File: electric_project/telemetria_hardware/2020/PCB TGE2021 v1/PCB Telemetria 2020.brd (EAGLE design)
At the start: 160 x 100 mm, 22 parts, among them IC1 INA240A1DR, IC2 MCP3221A6T-E_OTVAO, IC3 AZ1117IH-3.3TRG1, IC4 ACS758LCB-050B-PFF-T

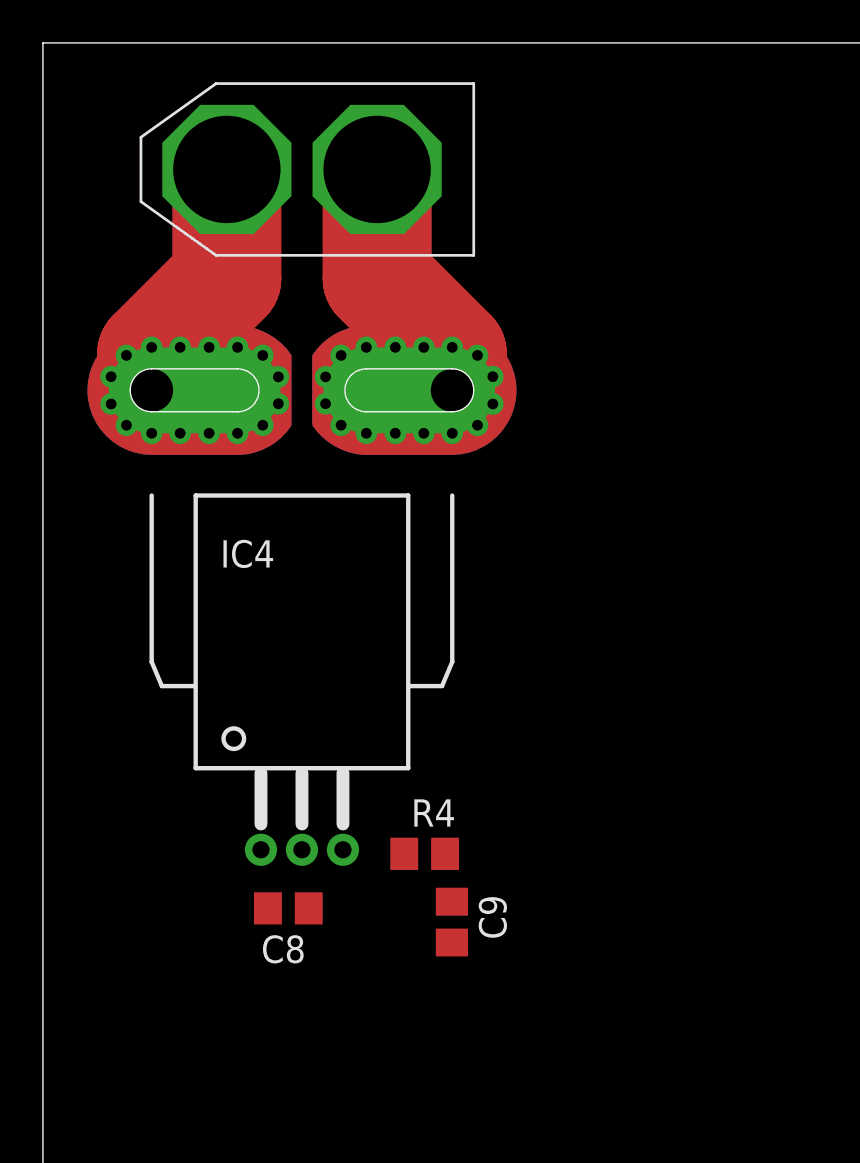
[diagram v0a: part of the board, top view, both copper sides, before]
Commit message: XT60 changes
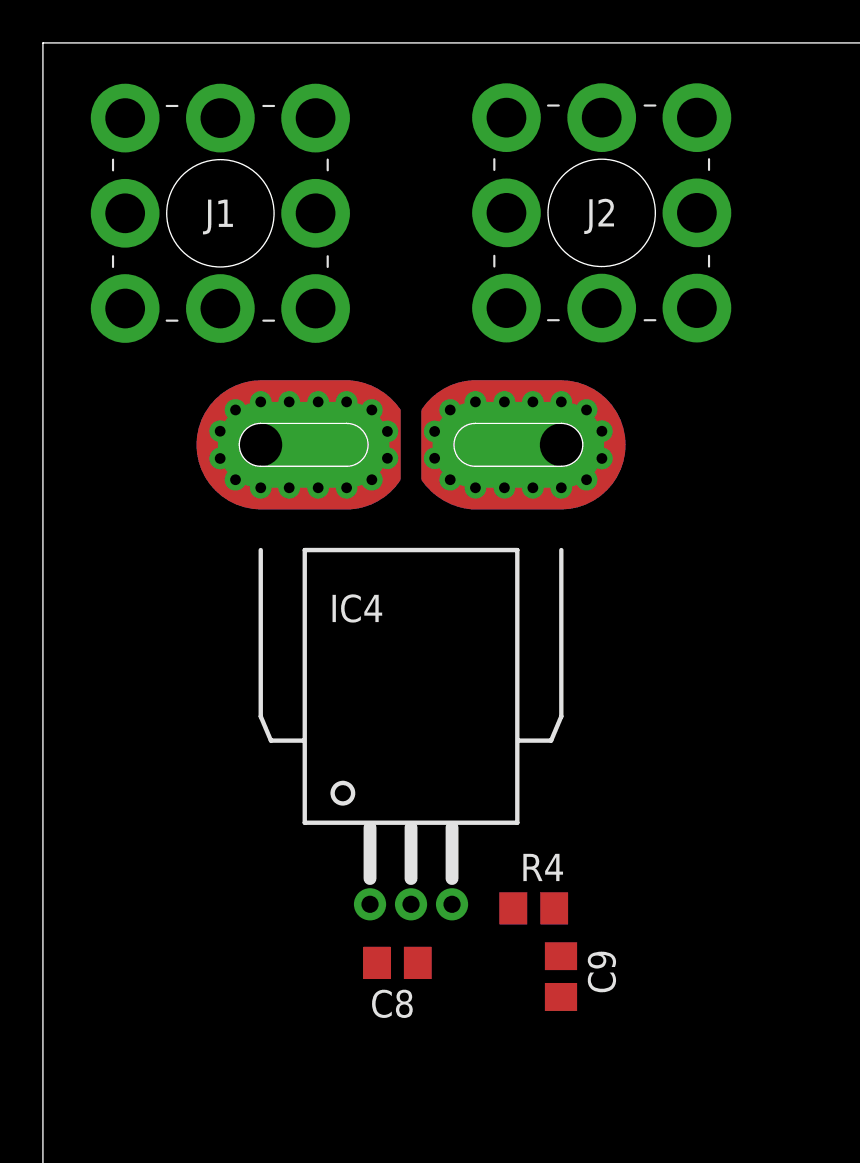
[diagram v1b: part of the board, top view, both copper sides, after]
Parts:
- removed U$3: XT60, XT60:XT60
- added J1, J2: 74655095R, SamacSys_Parts:74655095R
- moved C8 5.68 mm to (16.5, 57.1)
- moved C9 5.68 mm to (24.1, 56.5)
- moved R4 5.68 mm to (22.9, 59.7)
- moved IC4 5.68 mm to (17.1, 81.3)
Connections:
- net CMPPT_M: now also J1.1, J1.2, J1.3, J1.4, J1.5, J1.6, J1.7, J1.8; no longer U$3.-
- net CMPPT_P: now also J2.1, J2.2, J2.3, J2.4, J2.5, J2.6, J2.7, J2.8; no longer U$3.+
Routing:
- net CMPPT_M: track 11.7 -> 0.00 mm
- net CMPPT_P: track 11.7 -> 0.00 mm

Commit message: Adding XT60 documents
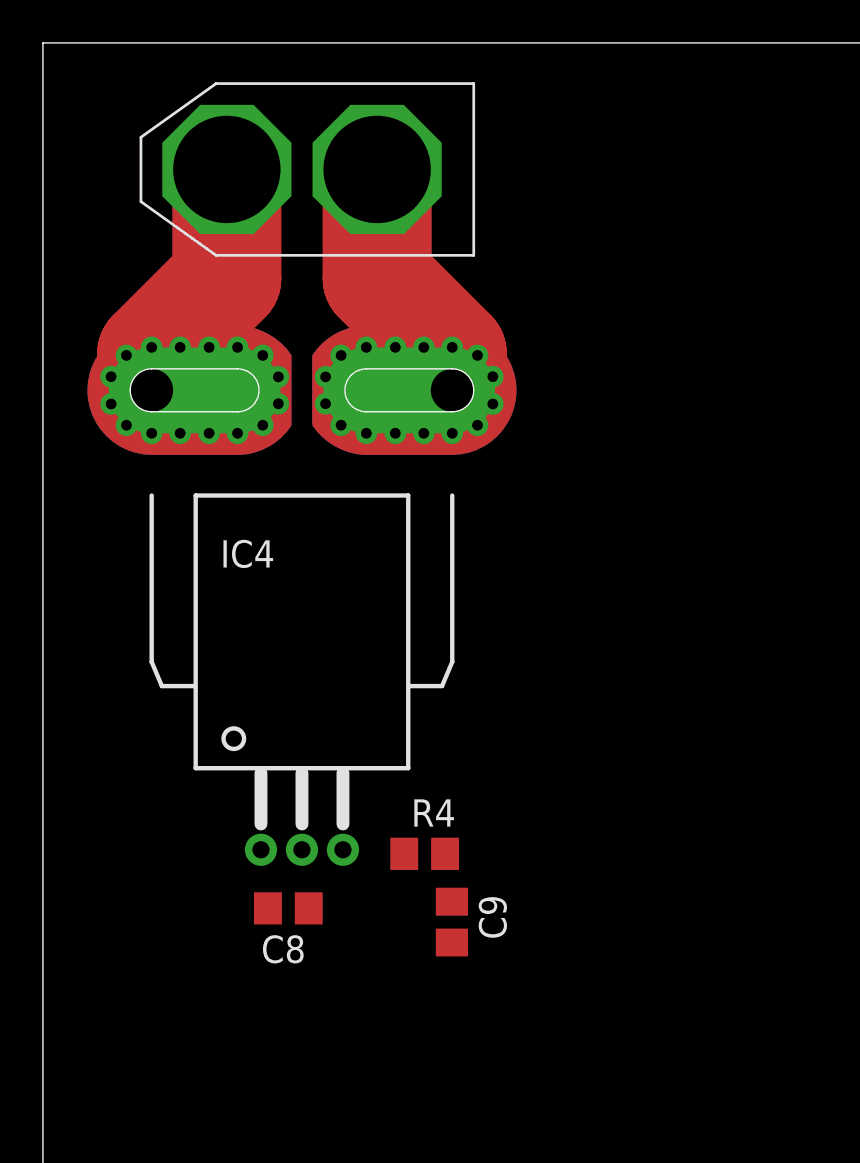
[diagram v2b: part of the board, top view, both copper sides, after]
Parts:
- removed J1, J2: 74655095R, SamacSys_Parts:74655095R
- added U$3: XT60, XT60:XT60
- moved C8 5.68 mm to (11.4, 59.7)
- moved C9 5.68 mm to (19.1, 59.1)
- moved R4 5.68 mm to (17.8, 62.2)
- moved IC4 5.68 mm to (12.1, 83.8)
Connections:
- net CMPPT_M: now also U$3.-; no longer J1.1, J1.2, J1.3, J1.4, J1.5, J1.6, J1.7, J1.8
- net CMPPT_P: now also U$3.+; no longer J2.1, J2.2, J2.3, J2.4, J2.5, J2.6, J2.7, J2.8
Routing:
- net CMPPT_M: track 0.00 -> 11.7 mm
- net CMPPT_P: track 0.00 -> 11.7 mm
